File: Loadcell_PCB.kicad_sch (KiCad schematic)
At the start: 53 parts, among them J1 USB_C_Receptacle_USB2.0, J2 Load cell side, J3 Micro_SD_Card, J4 GPS, Q1 S8550, SW1 RESET, U1 ATmega328P-M, U2 CH340C, U3 HX711, U4 74125, U5 LD1117S33TR_SOT223, Y1 16MHz

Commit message: Update unsaved record to the current commit
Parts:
- renumbered J4 to J2, J2 to J3, J3 to J4, R17 to R13, R13 to R14, R14 to R15, R15 to R16, R16 to R17, R6 to R5, R5 to R6
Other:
- moved on the sheet: C1, C10, C11, C12, C13, C14, C15, C2, C3, C4, C5, C6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

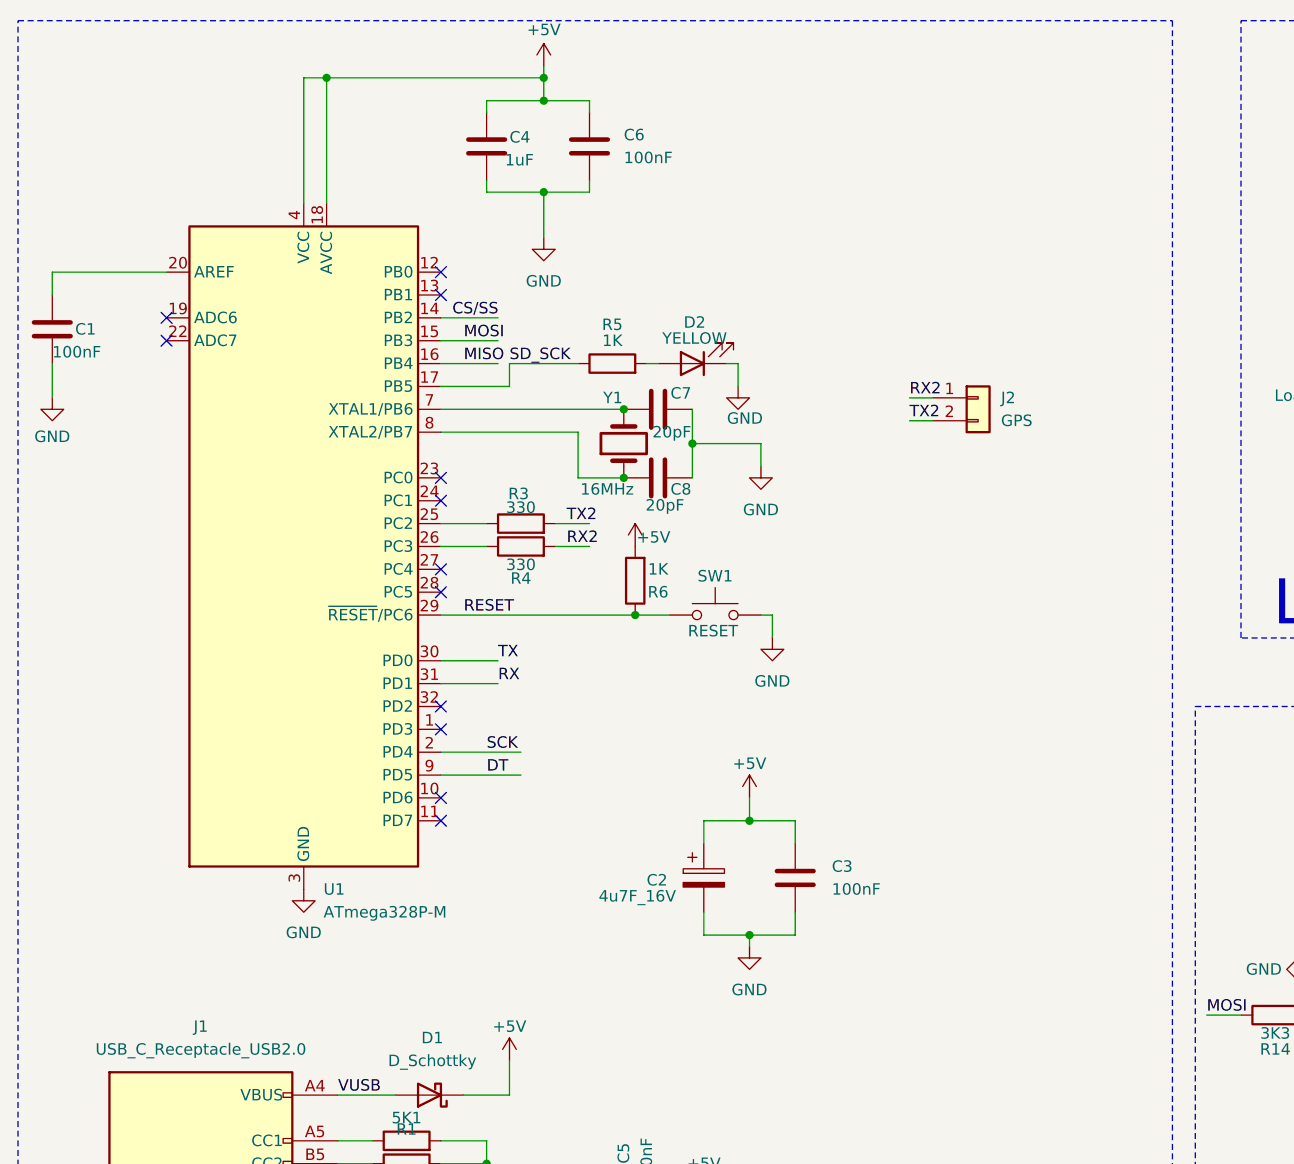
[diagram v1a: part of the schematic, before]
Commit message: Prepare for next revision - PT initial edit
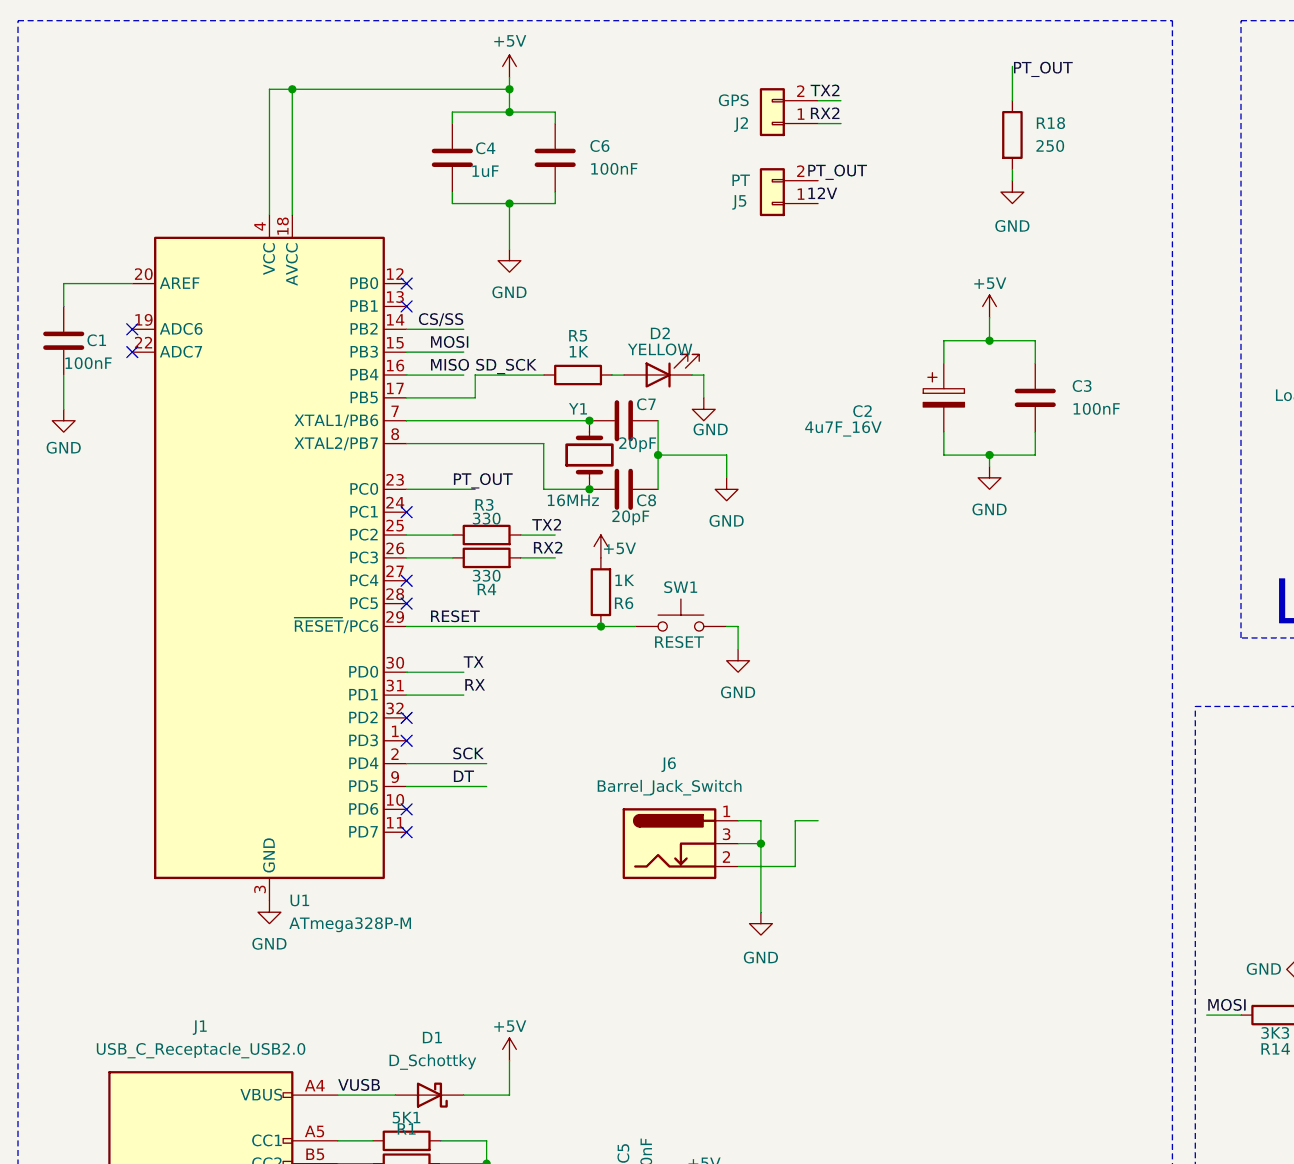
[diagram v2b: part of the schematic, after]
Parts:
- added J5: PT, Connector_PinHeader_2.54mm:PinHeader_1x02_P2.54mm_Horizontal, symbol Connector_Generic:Conn_01x02
- added J6: Barrel_Jack_Switch, symbol Connector:Barrel_Jack_Switch
- added R18: 250, Resistor_SMD:R_0805_2012Metric_Pad1.20x1.40mm_HandSolder, symbol Device:R
- J4: footprint Connector_Card:microSD_HC_Hirose_DM3BT-DSF-PEJS -> Connector_Card:microSD_HC_Molex_104031-0811
- U1: footprint Package_DFN_QFN:QFN-32-1EP_5x5mm_P0.5mm_EP3.1x3.1mm -> Package_QFP:TQFP-48-1EP_7x7mm_P0.5mm_EP5x5mm_ThermalVias
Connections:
- net GND: now also J6.1, J6.3, R18.2
- net PT_OUT: now reaches U1.23 (PC0)
- net PT_OUT: now also R18.1
- no-connect marks 23 -> 22
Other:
- moved on the sheet: C1, C2, C3, C4, C6, C7, C8, D2, J2, R3, R4, R5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
